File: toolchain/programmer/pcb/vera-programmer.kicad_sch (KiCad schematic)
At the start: 8 parts, among them J1 Conn_02x05_Odd_Even, SW1 SW_Push, U1 Pico

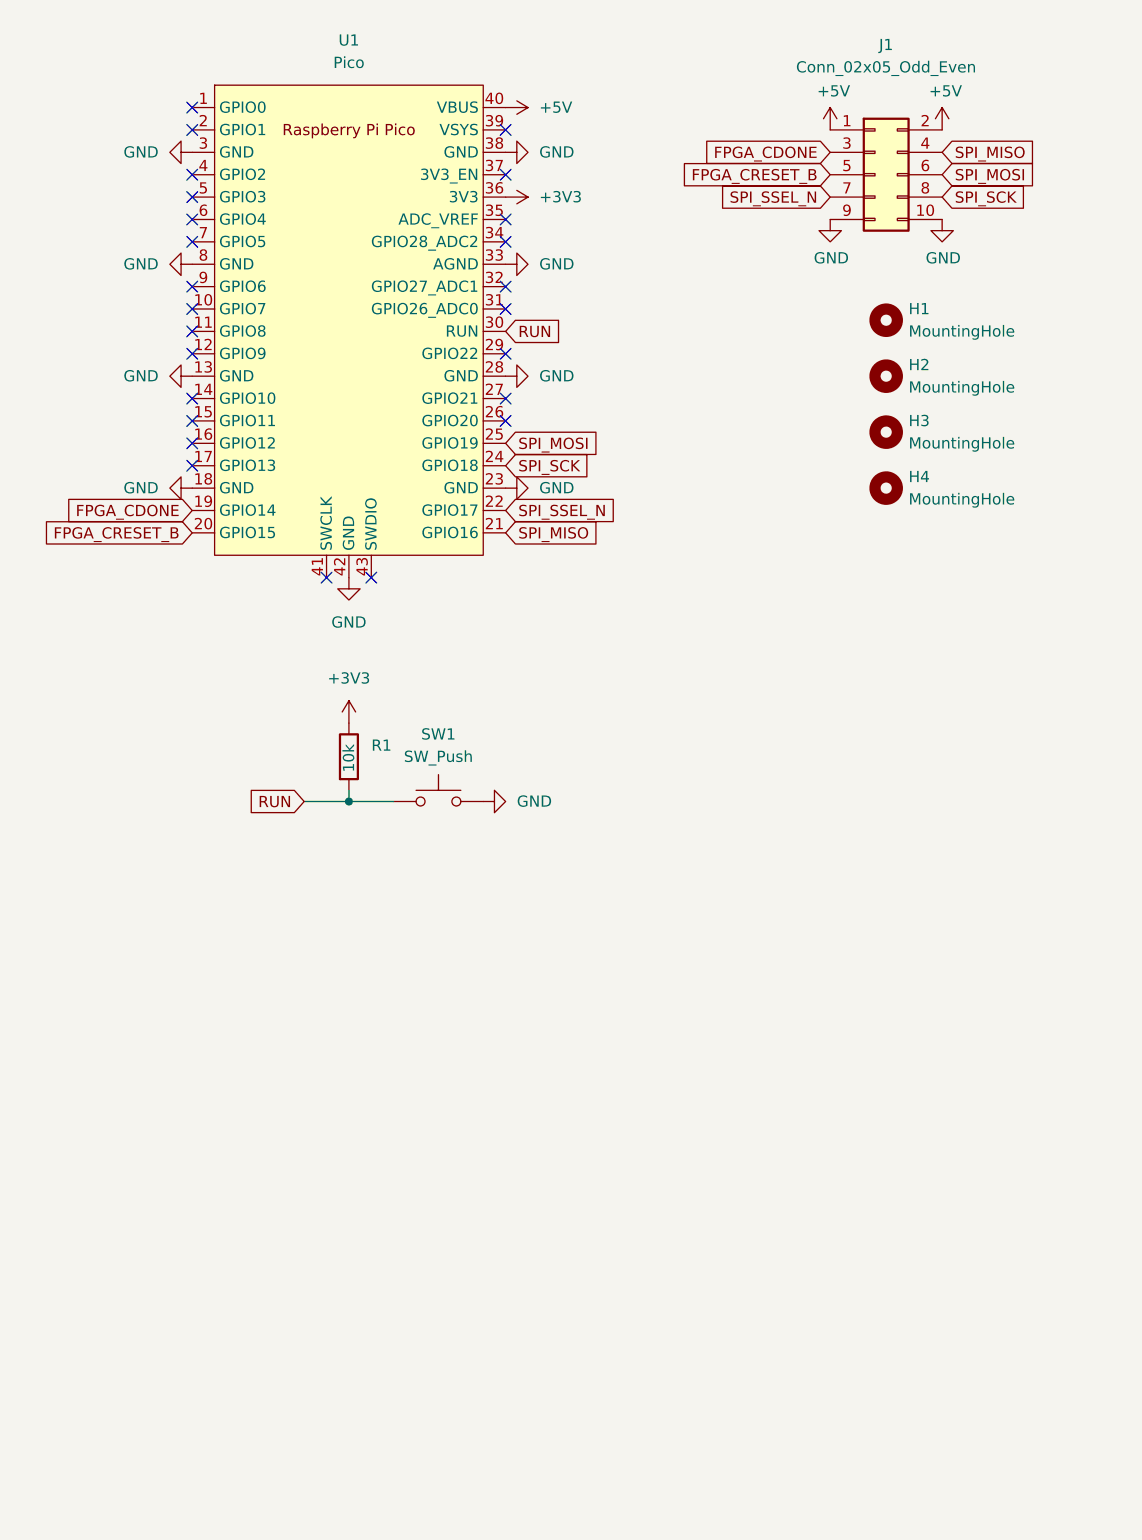
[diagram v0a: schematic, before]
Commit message: Fixing programmer board and updating licensing
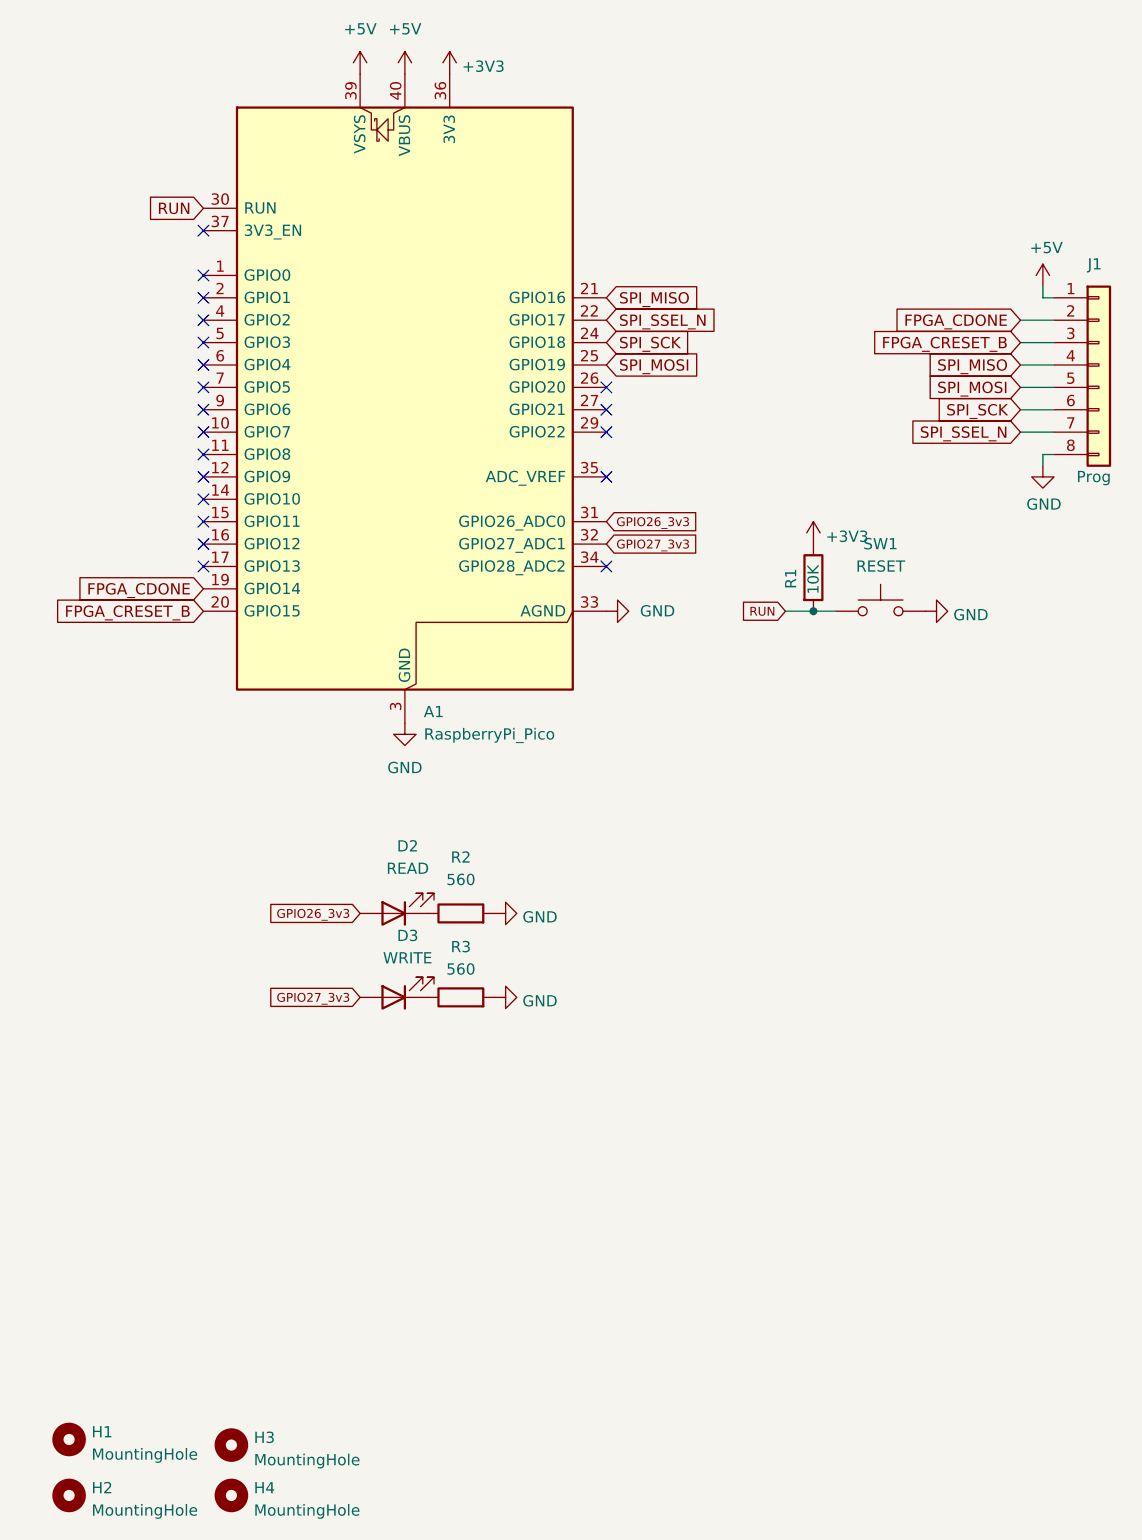
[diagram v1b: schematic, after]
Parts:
- removed J1: Conn_02x05_Odd_Even, Connector_IDC:IDC-Header_2x05_P2.54mm_Vertical, symbol Connector_Generic:Conn_02x05_Odd_Even
- removed U1: Pico, MCU_RaspberryPi_and_Boards:RPi_Pico_SMD_TH, symbol MCU_RaspberryPi_and_Boards:Pico
- added A1: RaspberryPi_Pico, Module:RaspberryPi_Pico_Common_Unspecified, symbol MCU_Module:RaspberryPi_Pico
- added D2: READ, LED_THT:LED_D5.0mm, symbol Device:LED
- added D3: WRITE, LED_THT:LED_D5.0mm, symbol Device:LED
- added J1: Prog, Connector_PinHeader_2.54mm:PinHeader_1x08_P2.54mm_Vertical, symbol Connector_Generic:Conn_01x08
- added R2, R3: 560, Resistor_THT:R_Axial_DIN0207_L6.3mm_D2.5mm_P7.62mm_Horizontal, symbol Device:R
- H1, H2, H3, H4: footprint MountingHole:MountingHole_3.2mm_M3_DIN965 -> MountingHole:MountingHole_3.2mm_M3; now in the parts list
- R1: value 10k -> 10K; LCSC (none) -> C17414; LCSC Part # (none) -> C17414
- SW1: value SW_Push -> RESET
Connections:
- net +3V3: now also A1.36 (3V3)
- net +5V: now also A1.39 (VSYS), A1.40 (VBUS), J1.1 (Pin_1)
- net FPGA_CDONE: now also A1.19 (GPIO14), J1.2 (Pin_2)
- net FPGA_CRESET_B: now also A1.20 (GPIO15), J1.3 (Pin_3)
- net GND: now also A1.13 (GND), A1.18 (GND), A1.23 (GND), A1.28 (GND), A1.3 (GND), A1.33 (AGND), A1.38 (GND), A1.8 (GND), J1.8 (Pin_8), R2.2, R3.2
- net RUN: now also A1.30 (RUN)
- net SPI_MISO: now also A1.21 (GPIO16), J1.4 (Pin_4)
- net SPI_MOSI: now also A1.25 (GPIO19), J1.5 (Pin_5)
- net SPI_SCK: now also A1.24 (GPIO18), J1.6 (Pin_6)
- net SPI_SSEL_N: now also A1.22 (GPIO17), J1.7 (Pin_7)
- new net: D3.1 (K), R3.1
- new net: D2.1 (K), R2.1
- new net GPIO26_3v3: A1.31 (GPIO26_ADC0), D2.2 (A)
- new net GPIO27_3v3: A1.32 (GPIO27_ADC1), D3.2 (A)
- no-connect marks 25 -> 20
